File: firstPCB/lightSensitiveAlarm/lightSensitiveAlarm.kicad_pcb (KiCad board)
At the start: 2 copper layers, 33 x 27.9 mm, 6 parts, among them Q1 BC547

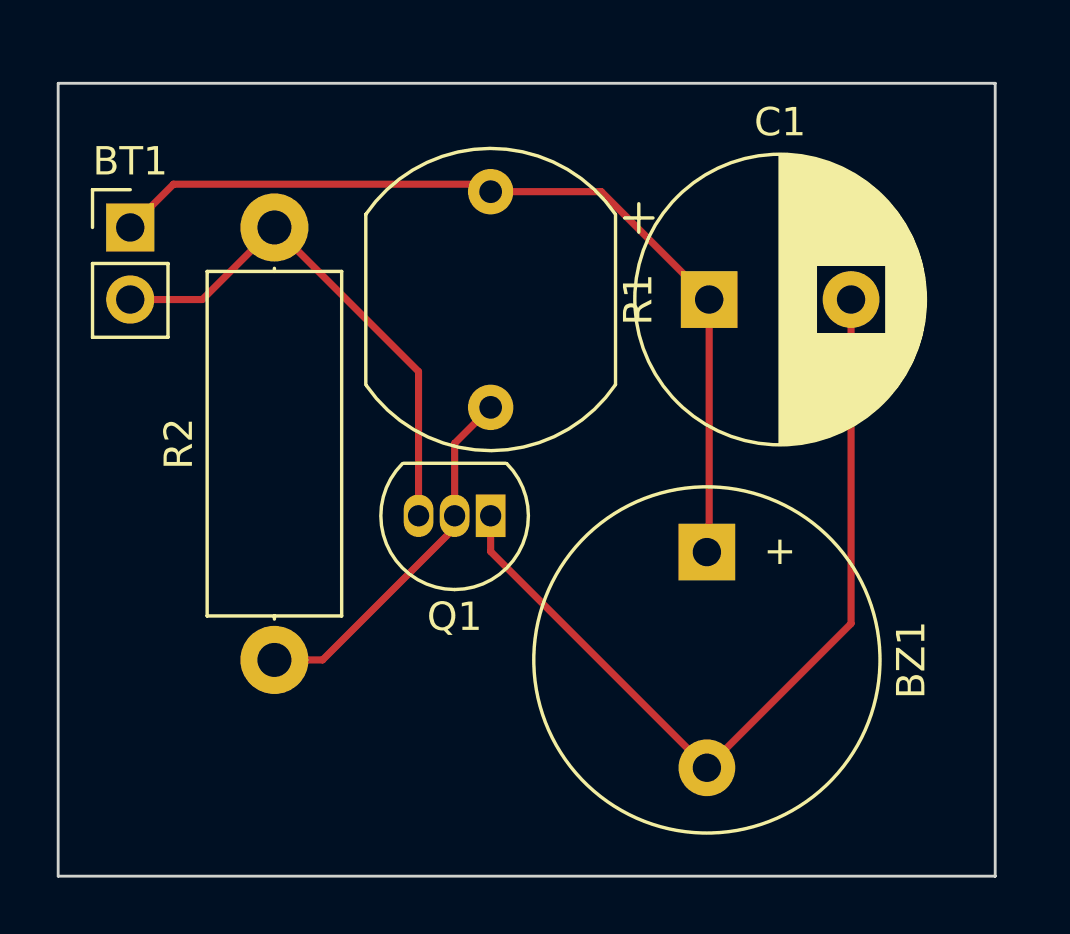
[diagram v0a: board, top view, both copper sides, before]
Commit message: mmmmmhm
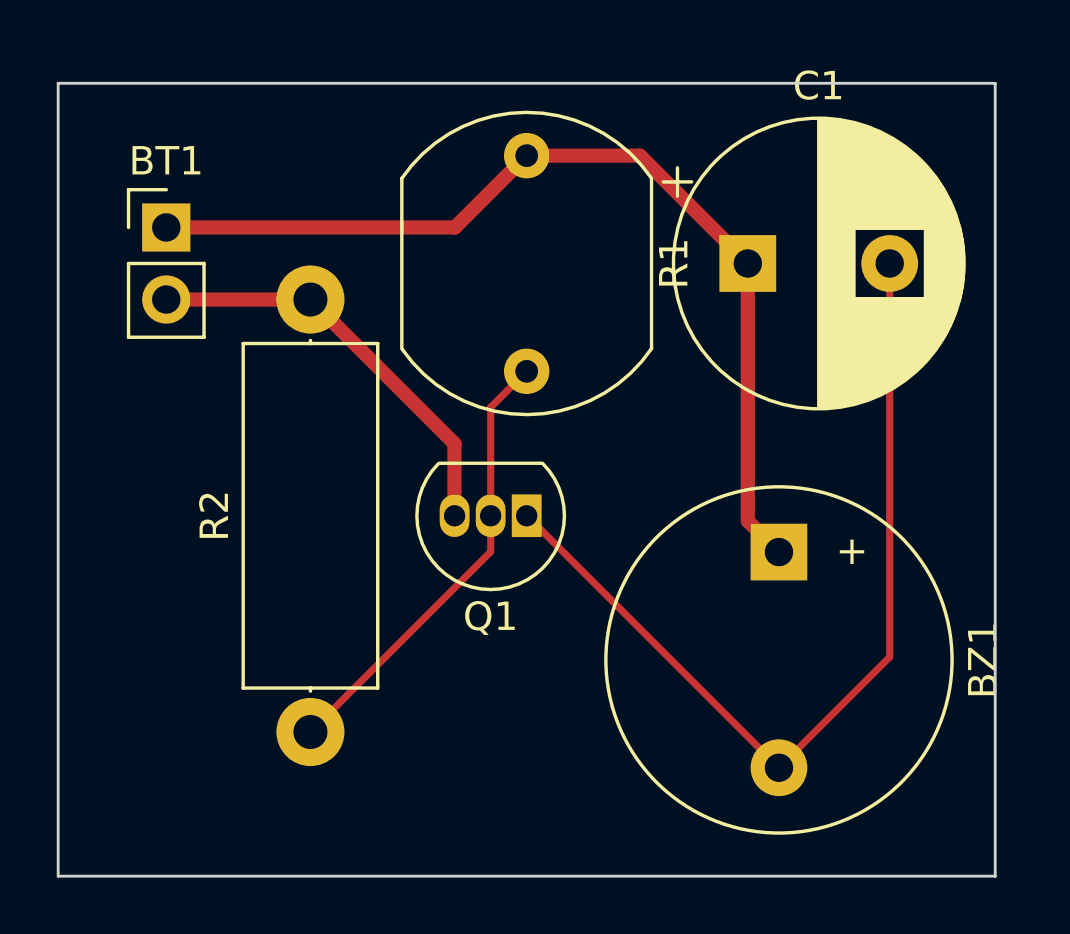
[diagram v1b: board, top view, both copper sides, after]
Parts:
- moved R2 2.84 mm to (92.7, 127.0)
- moved BZ1 2.54 mm to (109.2, 120.7)
- moved C1 1.86 mm to (108.1, 110.5)
- moved R1 1.80 mm to (100.3, 106.7)
- moved BT1 1.27 mm to (87.6, 109.2)
- moved Q1 1.27 mm to (100.3, 119.4)
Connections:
- net Net-(BT1-+) renamed /VCC
- net Net-(BT1--) renamed /Ground
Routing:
- net /Ground: track 18.4 -> 14.8 mm
- net Net-(Q1-B): track 13.1 -> 15.9 mm
- net /VCC: track 31.6 -> 33.7 mm
- net Net-(BZ1-+): track 30.6 -> 32.0 mm
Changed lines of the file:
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@@
   )
   (setup
+    (stackup
+      (layer "F.SilkS" (type "Top Silk Screen"))
+      (layer "F.Paste" (type "Top Solder Paste"))
+      (layer "F.Mask" (type "Top Solder Mask") (thickness 0.01))
+      (layer "F.Cu" (type "copper") (thickness 0.035))
+      (layer "dielectric 1" (type "core") (thickness 1.51) (material "FR4") (epsilon_r 4.5) (loss_tangent 0.02))
+      (layer "B.Cu" (type "copper") (thickness 0.035))
+      (layer "B.Mask" (type "Bottom Solder Mask") (thickness 0.01))
+      (layer "B.Paste" (type "Bottom Solder Paste"))
+      (layer "B.SilkS" (type "Bottom Silk Screen"))
+      (copper_finish "None")
+      (dielectric_constraints no)
+    )
     (pad_to_mask_clearance 0)
     (pcbplotparams
@@
   )
   (net 0 "")
-  (net 1 "Net-(BT1-+)")
-  (net 2 "Net-(BT1--)")
+  (net 1 "/VCC")
+  (net 2 "/Ground")
   (net 3 "Net-(BZ1-+)")
   (net 4 "Net-(Q1-B)")
   (footprint "Resistor_THT:R_Axial_DIN0414_L11.9mm_D4.5mm_P15.24mm_Horizontal" (layer "F.Cu")
-    (at 91.44 124.46 90)
+    (at 92.71 127 90)
     (descr "Resistor, Axial_DIN0414 series, Axial, Horizontal, pin pitch=15.24mm, 2W, length*diameter=11.9*4.5mm^2, http://www.vishay.com/docs/20128/wkxwrx.pdf")
     (tags "Resistor Axial_DIN0414 series Axial Horizontal pin pitch 15.24mm 2W length 11.9mm diameter 4.5mm")
@@
       (net 4 "Net-(Q1-B)") (pintype "passive"))
     (pad "2" thru_hole oval (at 15.24 0 90) (size 2.4 2.4) (drill 1.2) (layers "*.Cu" "*.Mask")
-      (net 2 "Net-(BT1--)") (pintype "passive"))
+      (net 2 "/Ground") (pintype "passive"))
     (model "${KICAD6_3DMODEL_DIR}/Resistor_THT.3dshapes/R_Axial_DIN0414_L11.9mm_D4.5mm_P15.24mm_Horizontal.wrl"
       (offset (xyz 0 0 0))
@@
   )
   (footprint "OptoDevice:R_LDR_10x8.5mm_P7.6mm_Vertical" (layer "F.Cu")
-    (at 99.06 107.96 -90)
+    (at 100.33 106.69 -90)
     (descr "Resistor, LDR 10x8.5mm")
     (tags "Resistor LDR10.8.5mm")
@@
       (stroke (width 0.1) (type solid)) (layer "F.Fab"))
     (pad "1" thru_hole circle (at 0 0 270) (size 1.6 1.6) (drill 0.8) (layers "*.Cu" "*.Mask")
-      (net 1 "Net-(BT1-+)") (pintype "passive"))
+      (net 1 "/VCC") (pintype "passive"))
     (pad "2" thru_hole circle (at 7.6 0 270) (size 1.6 1.6) (drill 0.8) (layers "*.Cu" "*.Mask")
       (net 4 "Net-(Q1-B)") (pintype "passive"))
@@
   )
   (footprint "Connector_PinHeader_2.54mm:PinHeader_1x02_P2.54mm_Vertical" (layer "F.Cu")
-    (at 86.36 109.22)
+    (at 87.63 109.22)
     (descr "Through hole straight pin header, 1x02, 2.54mm pitch, single row")
     (tags "Through hole pin header THT 1x02 2.54mm single row")
@@
       (stroke (width 0.1) (type solid)) (layer "F.Fab"))
     (pad "1" thru_hole rect (at 0 0) (size 1.7 1.7) (drill 1) (layers "*.Cu" "*.Mask")
-      (net 1 "Net-(BT1-+)") (pinfunction "+") (pintype "passive"))
+      (net 1 "/VCC") (pinfunction "+") (pintype "passive"))
     (pad "2" thru_hole oval (at 0 2.54) (size 1.7 1.7) (drill 1) (layers "*.Cu" "*.Mask")
-      (net 2 "Net-(BT1--)") (pinfunction "-") (pintype "passive"))
+      (net 2 "/Ground") (pinfunction "-") (pintype "passive"))
     (model "${KICAD6_3DMODEL_DIR}/Connector_PinHeader_2.54mm.3dshapes/PinHeader_1x02_P2.54mm_Vertical.wrl"
       (offset (xyz 0 0 0))
@@
   )
   (footprint "Package_TO_SOT_THT:TO-92_Inline" (layer "F.Cu")
-    (at 99.06 119.38 180)
+    (at 100.33 119.38 180)
     (descr "TO-92 leads in-line, narrow, oval pads, drill 0.75mm (see NXP sot054_po.pdf)")
     (tags "to-92 sc-43 sc-43a sot54 PA33 transistor")
@@
       (net 4 "Net-(Q1-B)") (pinfunction "B") (pintype "input"))
     (pad "3" thru_hole oval (at 2.54 0 180) (size 1.05 1.5) (drill 0.75) (layers "*.Cu" "*.Mask")
-      (net 2 "Net-(BT1--)") (pinfunction "E") (pintype "passive"))
+      (net 2 "/Ground") (pinfunction "E") (pintype "passive"))
     (model "${KICAD6_3DMODEL_DIR}/Package_TO_SOT_THT.3dshapes/TO-92_Inline.wrl"
       (offset (xyz 0 0 0))
@@
   )
   (footprint "Buzzer_Beeper:Buzzer_12x9.5RM7.6" (layer "F.Cu")
-    (at 106.68 120.66 -90)
+    (at 109.22 120.66 -90)
     (descr "Generic Buzzer, D12mm height 9.5mm with RM7.6mm")
     (tags "buzzer")
@@
       (stroke (width 0.1) (type solid)) (fill none) (layer "F.Fab"))
     (pad "1" thru_hole rect (at 0 0 270) (size 2 2) (drill 1) (layers "*.Cu" "*.Mask")
-      (net 1 "Net-(BT1-+)") (pinfunction "-") (pintype "passive"))
+      (net 1 "/VCC") (pinfunction "-") (pintype "passive"))
     (pad "2" thru_hole circle (at 7.6 0 270) (size 2 2) (drill 1) (layers "*.Cu" "*.Mask")
       (net 3 "Net-(BZ1-+)") (pinfunction "+") (pintype "passive"))
@@
   )
   (footprint "Capacitor_THT:CP_Radial_D10.0mm_P5.00mm" (layer "F.Cu")
-    (at 106.76 111.76)
+    (at 108.122323 110.49)
     (descr "CP, Radial series, Radial, pin pitch=5.00mm, , diameter=10mm, Electrolytic Capacitor")
     (tags "CP Radial series Radial pin pitch 5.00mm  diameter 10mm Electrolytic Capacitor")
@@
       (stroke (width 0.1) (type solid)) (fill none) (layer "F.Fab"))
     (pad "1" thru_hole rect (at 0 0) (size 2 2) (drill 1) (layers "*.Cu" "*.Mask")
-      (net 1 "Net-(BT1-+)") (pintype "passive"))
+      (net 1 "/VCC") (pintype "passive"))
     (pad "2" thru_hole circle (at 5 0) (size 2 2) (drill 1) (layers "*.Cu" "*.Mask")
       (net 3 "Net-(BZ1-+)") (pintype "passive"))
@@
   (gr_rect (start 83.82 104.14) (end 116.84 132.08)
     (stroke (width 0.1) (type default)) (fill none) (layer "Edge.Cuts"))
-  (segment (start 98.795 107.695) (end 99.06 107.96) (width 0.25) (layer "F.Cu") (net 1))
-  (segment (start 87.885 107.695) (end 98.795 107.695) (width 0.25) (layer "F.Cu") (net 1))
-  (segment (start 102.96 107.96) (end 106.76 111.76) (width 0.25) (layer "F.Cu") (net 1))
-  (segment (start 86.36 109.22) (end 87.885 107.695) (width 0.25) (layer "F.Cu") (net 1))
-  (segment (start 99.06 107.96) (end 102.96 107.96) (width 0.25) (layer "F.Cu") (net 1))
-  (segment (start 106.76 111.76) (end 106.76 120.58) (width 0.25) (layer "F.Cu") (net 1))
-  (segment (start 106.76 120.58) (end 106.68 120.66) (width 0.25) (layer "F.Cu") (net 1))
-  (segment (start 96.52 114.3) (end 91.44 109.22) (width 0.25) (layer "F.Cu") (net 2))
-  (segment (start 96.52 119.38) (end 96.52 114.3) (width 0.25) (layer "F.Cu") (net 2))
-  (segment (start 91.44 109.22) (end 88.9 111.76) (width 0.25) (layer "F.Cu") (net 2))
-  (segment (start 88.9 111.76) (end 86.36 111.76) (width 0.25) (layer "F.Cu") (net 2))
-  (segment (start 111.76 111.76) (end 111.76 123.18) (width 0.25) (layer "F.Cu") (net 3))
-  (segment (start 99.06 120.64) (end 99.06 119.38) (width 0.25) (layer "F.Cu") (net 3))
-  (segment (start 111.76 123.18) (end 106.68 128.26) (width 0.25) (layer "F.Cu") (net 3))
-  (segment (start 106.68 128.26) (end 99.06 120.64) (width 0.25) (layer "F.Cu") (net 3))
-  (segment (start 91.44 124.46) (end 93.137056 124.46) (width 0.25) (layer "F.Cu") (net 4))
-  (segment (start 97.79 119.807056) (end 97.79 119.38) (width 0.25) (layer "F.Cu") (net 4))
-  (segment (start 97.79 116.83) (end 97.79 119.38) (width 0.25) (layer "F.Cu") (net 4))
-  (segment (start 99.06 115.56) (end 97.79 116.83) (width 0.25) (layer "F.Cu") (net 4))
-  (segment (start 93.137056 124.46) (end 97.79 119.807056) (width 0.25) (layer "F.Cu") (net 4))
+  (segment (start 87.63 109.22) (end 97.8 109.22) (width 0.5) (layer "F.Cu") (net 1))
+  (segment (start 97.8 109.22) (end 100.33 106.69) (width 0.5) (layer "F.Cu") (net 1))
+  (segment (start 100.33 106.69) (end 104.322323 106.69) (width 0.5) (layer "F.Cu") (net 1))
+  (segment (start 108.122323 119.562323) (end 109.22 120.66) (width 0.5) (layer "F.Cu") (net 1))
+  (segment (start 108.122323 110.49) (end 108.122323 119.562323) (width 0.5) (layer "F.Cu") (net 1))
+  (segment (start 104.322323 106.69) (end 108.122323 110.49) (width 0.5) (layer "F.Cu") (net 1))
+  (segment (start 87.63 111.76) (end 92.71 111.76) (width 0.5) (layer "F.Cu") (net 2))
+  (segment (start 97.785 116.835) (end 97.785 119.38) (width 0.5) (layer "F.Cu") (net 2))
+  (segment (start 92.71 111.76) (end 97.785 116.835) (width 0.5) (layer "F.Cu") (net 2))
+  (segment (start 109.22 128.26) (end 113.122323 124.357677) (width 0.25) (layer "F.Cu") (net 3))
+  (segment (start 113.122323 124.357677) (end 113.122323 110.49) (width 0.25) (layer "F.Cu") (net 3))
+  (segment (start 100.33 119.38) (end 100.34 119.38) (width 0.25) (layer "F.Cu") (net 3))
+  (segment (start 100.34 119.38) (end 109.22 128.26) (width 0.25) (layer "F.Cu") (net 3))
+  (segment (start 99.06 119.38) (end 99.06 115.56) (width 0.25) (layer "F.Cu") (net 4))
+  (segment (start 99.06 119.38) (end 99.06 120.65) (width 0.25) (layer "F.Cu") (net 4))
+  (segment (start 99.06 115.56) (end 100.33 114.29) (width 0.25) (layer "F.Cu") (net 4))
+  (segment (start 99.06 120.65) (end 92.71 127) (width 0.25) (layer "F.Cu") (net 4))
 )
